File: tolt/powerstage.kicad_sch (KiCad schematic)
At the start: 72 parts, among them Q1 NMOS, Q10 NMOS, Q11 NMOS, Q12 NMOS, Q13 NMOS, Q14 NMOS, Q15 NMOS, Q16 NMOS, Q17 NMOS, Q18 NMOS, Q2 NMOS, Q3 NMOS, Q4 NMOS, Q5 NMOS, Q6 NMOS, Q7 NMOS, Q8 NMOS, Q9 NMOS

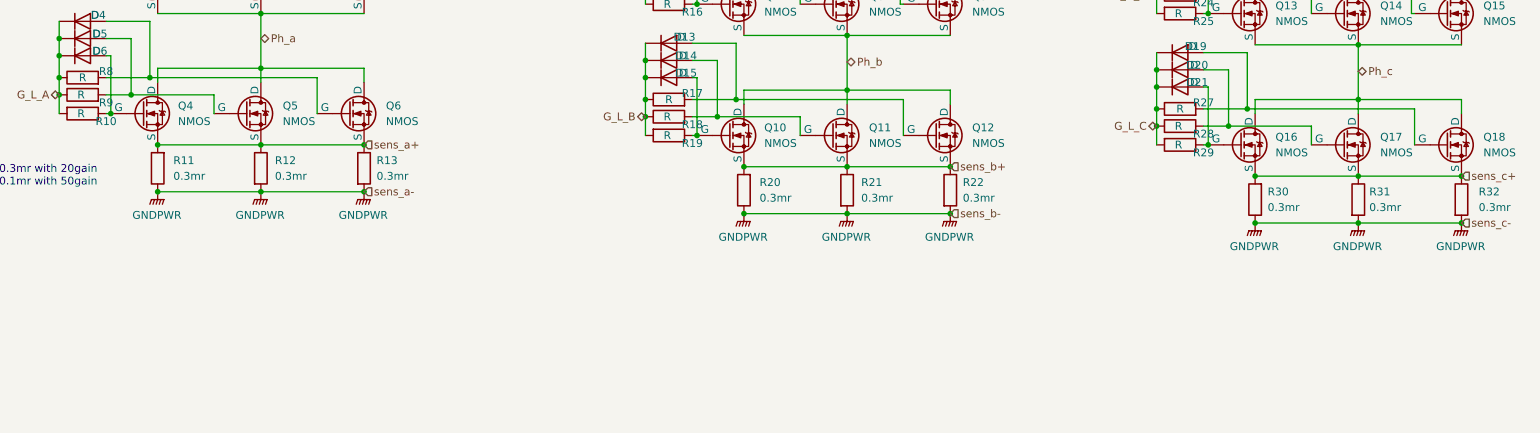
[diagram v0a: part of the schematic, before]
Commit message: new file:   tolt/Library.pretty/IND-SMD_L3.9-W3.9-1.kicad_mod 	new file:   tolt/Library.pretty/IND-SMD_L5.0-W5.0.kicad_mod 	modified:   tolt/auxl.kicad_sch 	modified:   tolt/conn.kicad_sch 	modified:   tolt/converters.kicad_sch 	new file:   tolt/fp-lib-table 	modified:   tolt/inter.kicad_sch 	modified:   tolt/powerstage.kicad_sch 	modified:   tolt/stm32.kicad_sch 	modified:   tolt/tolt.kicad_sch
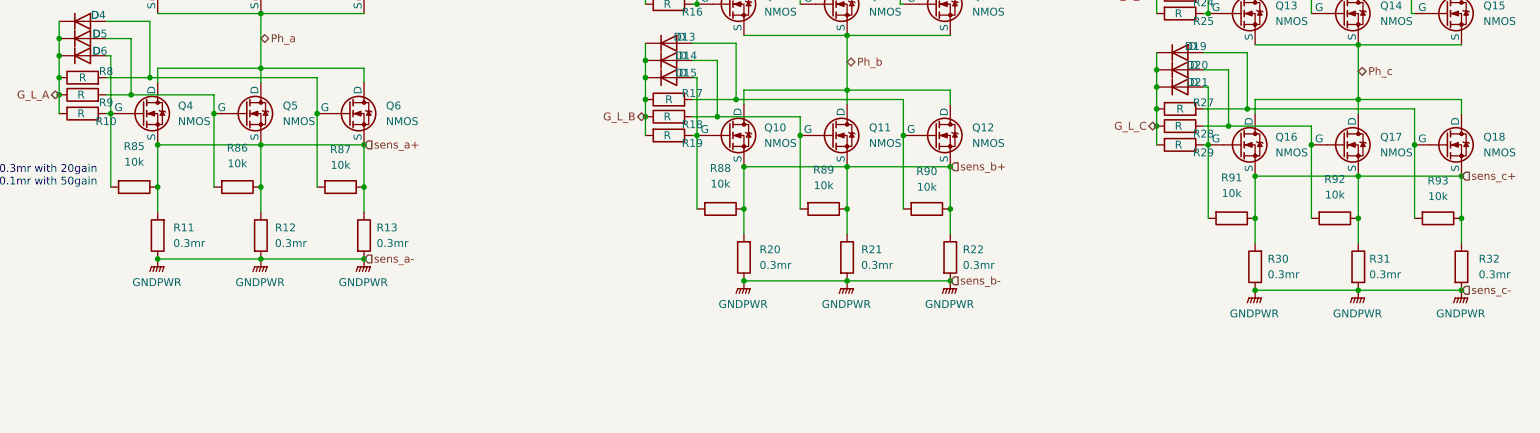
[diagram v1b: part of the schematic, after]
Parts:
- added R85, R86, R87, R88, R89, R90, R91, R92, R93: 10k, Resistor_SMD:R_0603_1608Metric, symbol Device:R
- D10, D11, D12, D13, D14, D15, D16, D17, D18, D19, D20, D21, D6, D7, D8, D9: footprint (none) -> Diode_SMD:D_SOD-123
- D4, D5: footprint (none) -> Diode_SMD:D_SOD-123F
- R10, R14, R15, R16, R17, R18, R19, R23, R24, R25, R27, R28, R29, R5, R6, R7, R8, R9: footprint (none) -> Resistor_SMD:R_0805_2012Metric_Pad1.20x1.40mm_HandSolder
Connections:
- net sens_a+: now also R85.1, R86.1, R87.1
- net sens_b+: now also R88.1, R89.1, R90.1
- net sens_c+: now also R91.1, R92.1, R93.1
- net at D20.2 (A), Q17.2 (G), R28.2: now also R92.2
- net at D6.2 (A), Q4.2 (G), R10.1: now also R85.2
- net at D14.2 (A), Q11.2 (G), R18.2: now also R89.2
- net at D15.2 (A), Q10.2 (G), R19.1: now also R88.2
- net at D21.2 (A), Q16.2 (G), R29.1: now also R91.2
- net at D19.2 (A), Q18.2 (G), R27.2: now also R93.2
- net at D13.2 (A), Q12.2 (G), R17.2: now also R90.2
- net at D4.2 (A), Q6.2 (G), R8.2: now also R87.2
- net at D5.2 (A), Q5.2 (G), R9.2: now also R86.2
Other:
- moved on the sheet: R11, R12, R13, R20, R21, R22, R30, R31, R32

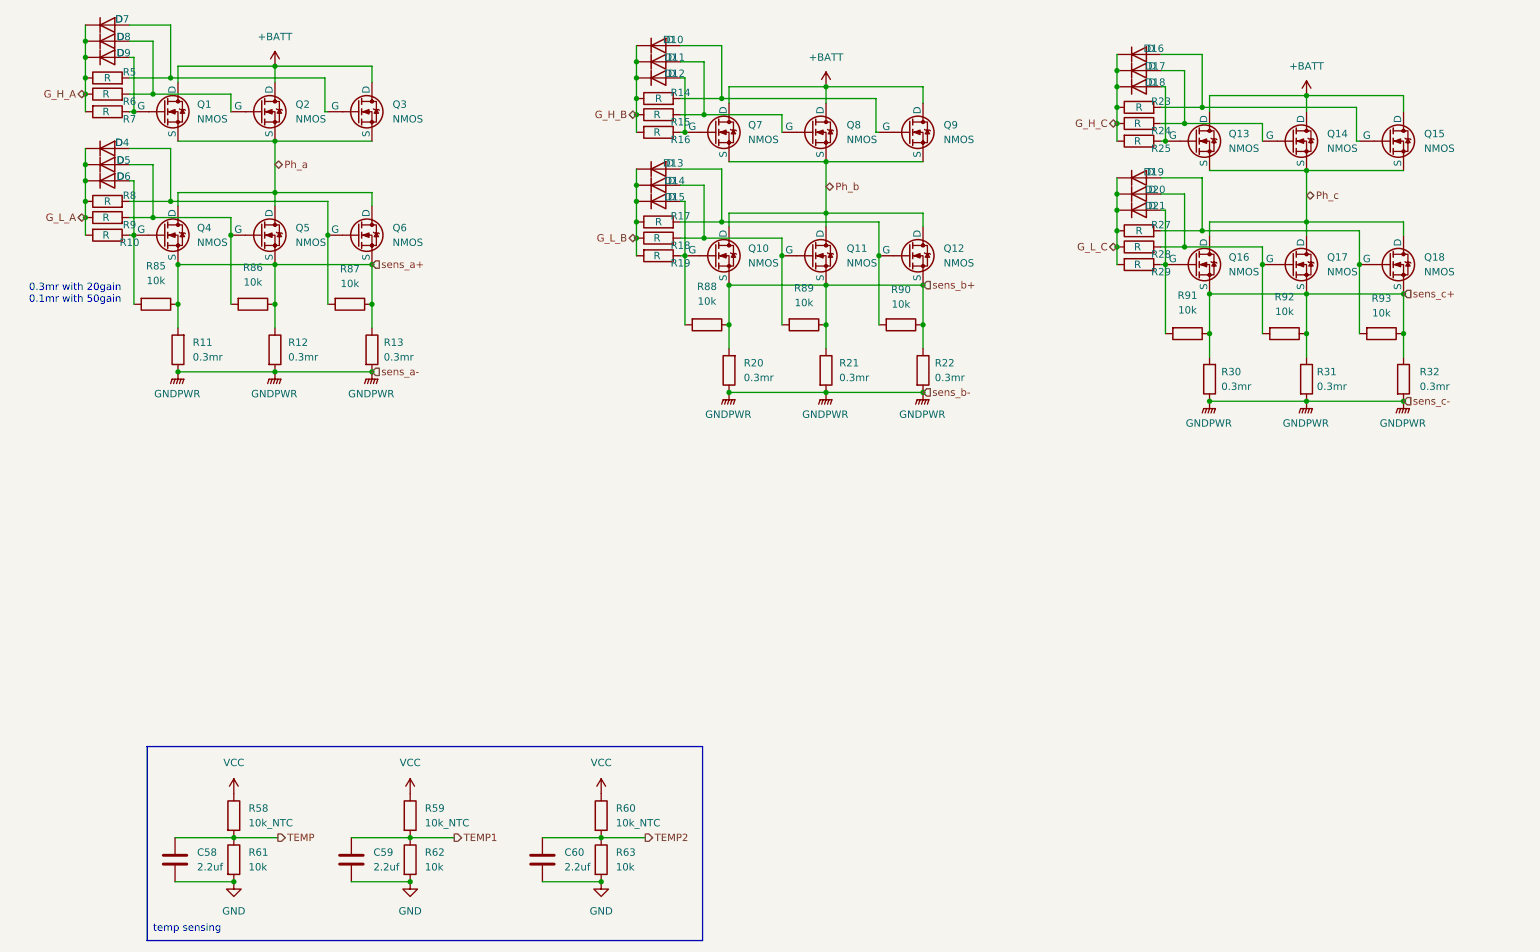
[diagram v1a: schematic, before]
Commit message: new file:   tolt/Library.pretty/PQDE6W.kicad_mod 	modified:   tolt/auxl.kicad_sch 	modified:   tolt/conn.kicad_sch 	modified:   tolt/converters.kicad_sch 	modified:   tolt/powerstage.kicad_sch 	modified:   tolt/tolt.kicad_pcb 	modified:   tolt/tolt.kicad_sch
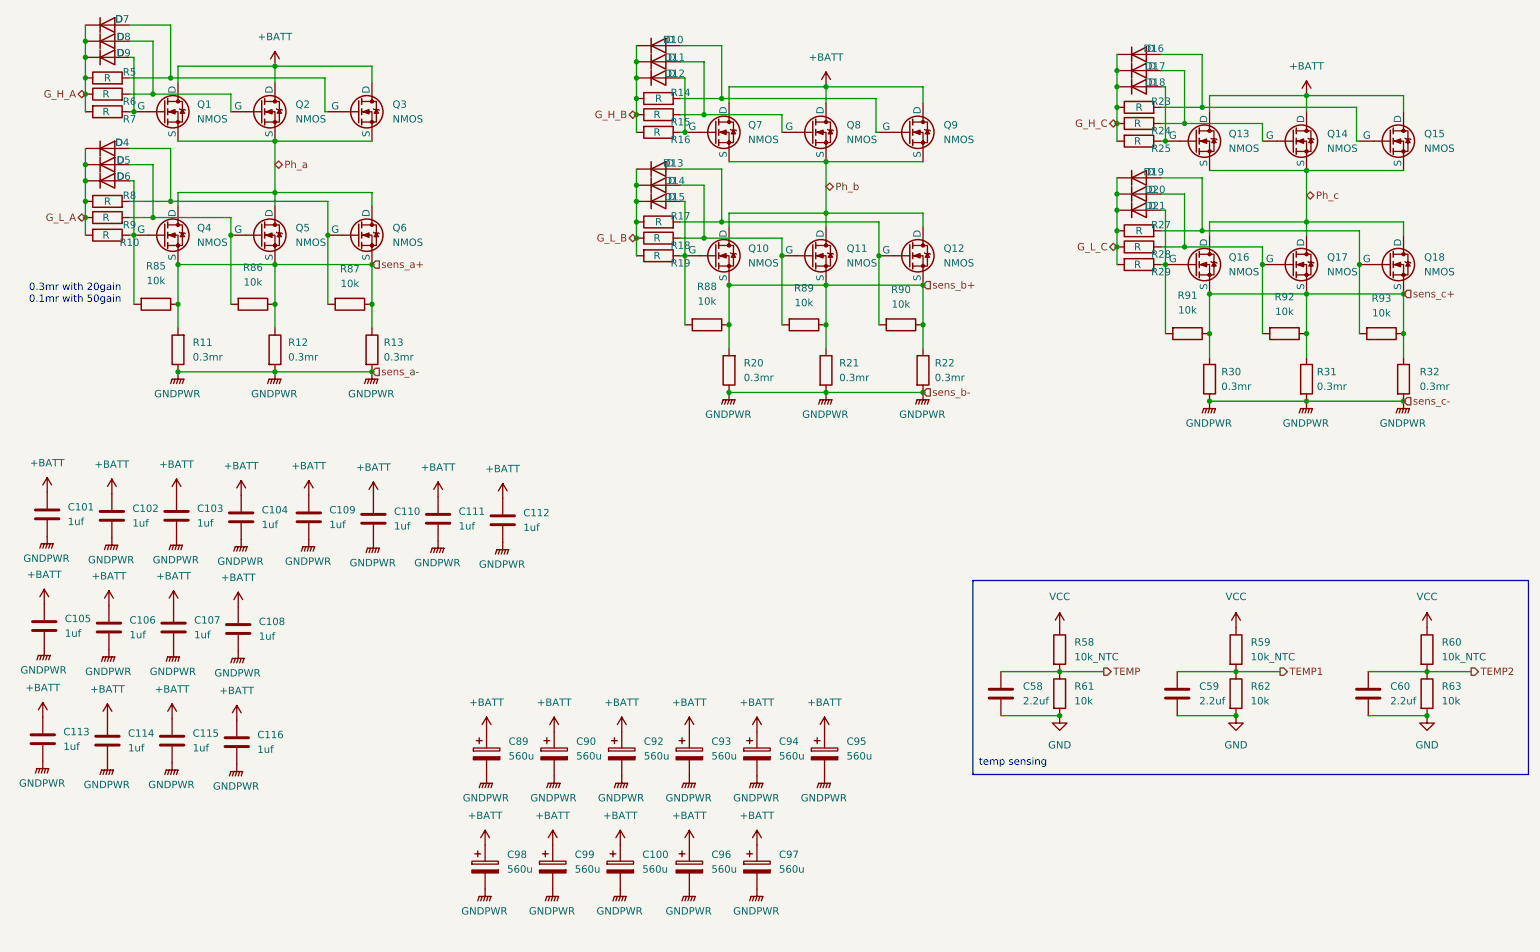
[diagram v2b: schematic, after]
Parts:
- added C100, C89, C90, C92, C93, C94, C95, C96, C97, C98, C99: 560u, Capacitor_THT:CP_Radial_D16.0mm_P7.50mm, symbol Device:C_Polarized
- added C101, C102, C103, C104, C105, C106, C107, C108, C109, C110, C111, C112, C113, C114, C115, C116: 1uf, Capacitor_SMD:C_2220_5750Metric_Pad1.97x5.40mm_HandSolder, symbol Device:C
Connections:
- net +BATT: now also C100.1, C101.1, C102.1, C103.1, C104.1, C105.1, C106.1, C107.1, C108.1, C109.1, C110.1, C111.1, C112.1, C113.1, C114.1, C115.1, C116.1, C89.1, C90.1, C92.1, C93.1, C94.1, C95.1, C96.1, C97.1, C98.1, C99.1
- net GNDPWR: now also C100.2, C101.2, C102.2, C103.2, C104.2, C105.2, C106.2, C107.2, C108.2, C109.2, C110.2, C111.2, C112.2, C113.2, C114.2, C115.2, C116.2, C89.2, C90.2, C92.2, C93.2, C94.2, C95.2, C96.2, C97.2, C98.2, C99.2
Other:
- moved on the sheet: C58, C59, C60, R58, R59, R60, R61, R62, R63
